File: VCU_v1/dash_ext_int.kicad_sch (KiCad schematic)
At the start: 33 parts, among them U15 SP8K80TB1, U16 SP8K80TB1

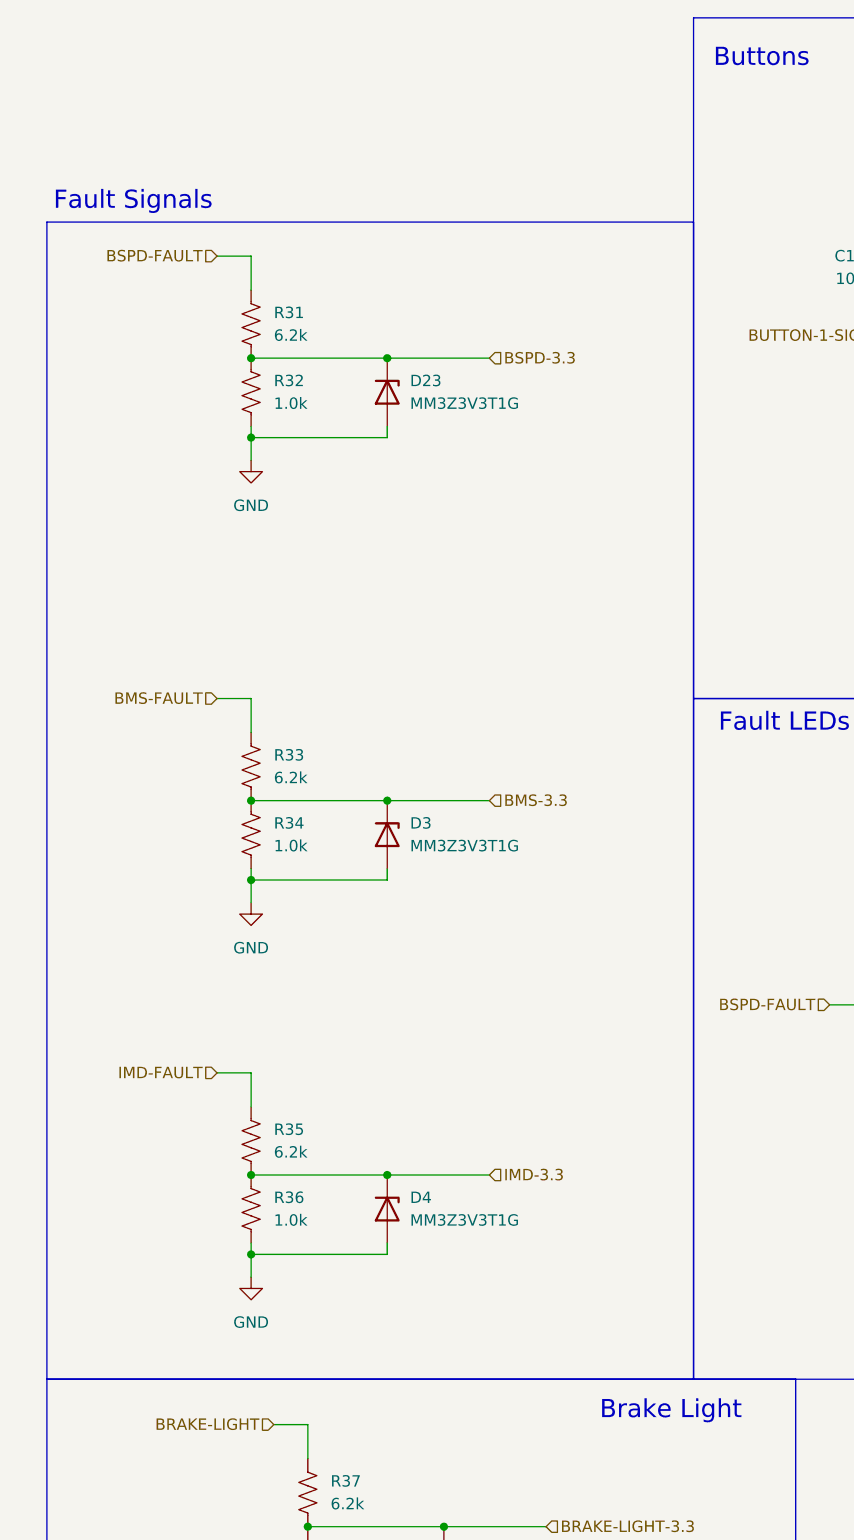
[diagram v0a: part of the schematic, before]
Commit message: left to do before layout: wire DRS/Debug LEDs to connector, add BRUHbus ports
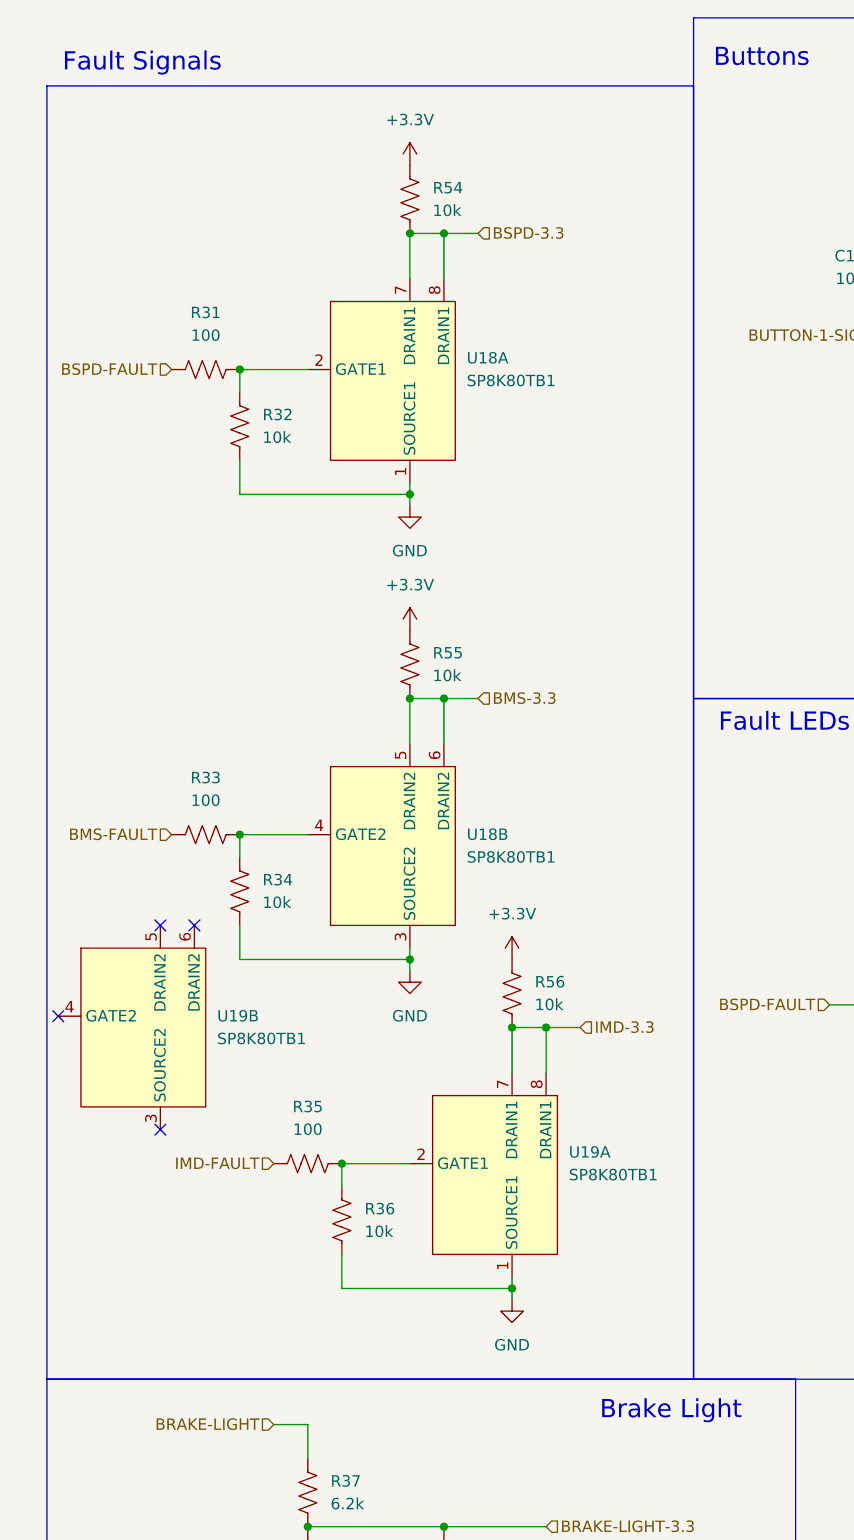
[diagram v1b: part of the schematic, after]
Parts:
- removed D23, D3, D4: MM3Z3V3T1G, Diode_SMD:D_SOD-323_HandSoldering, symbol .Diode-Zener:MM3Z3V3T1G
- removed R31, R33, R35: 6.2k, Resistor_SMD:R_0603_1608Metric_Pad0.98x0.95mm_HandSolder, symbol BFR Resistors:RMCF0603FT6K20
- removed R32, R34, R36: 1.0k, Resistor_SMD:R_0603_1608Metric_Pad0.98x0.95mm_HandSolder, symbol BFR Resistors:RMCF0603FT1K00
- added R31, R33, R35: 100, Resistor_SMD:R_0603_1608Metric_Pad0.98x0.95mm_HandSolder, symbol BFR Resistors:RMCF0603FT100R
- added R32, R34, R36, R54, R55, R56: 10k, Resistor_SMD:R_0603_1608Metric_Pad0.98x0.95mm_HandSolder, symbol BFR Resistors:RMCF0603FT10K0
- added U18, U19: SP8K80TB1, symbol SP8KK80TB1:SP8K80TB1
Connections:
- net BMS-3.3: now also R55.1, U18.5 (DRAIN2), U18.6 (DRAIN2)
- net BMS-FAULT: now also R33.1
- net BSPD-3.3: now also R54.1, U18.7 (DRAIN1), U18.8 (DRAIN1)
- net BSPD-FAULT: now also R31.1
- net GND: now also R32.1, R34.1, R36.1, U18.1 (SOURCE1), U18.3 (SOURCE2), U19.1 (SOURCE1)
- net IMD-3.3: now also R56.1, U19.7 (DRAIN1), U19.8 (DRAIN1)
- net IMD-FAULT: now also R35.1
- new net: R33.2, R34.2, U18.4 (GATE2)
- new net: R31.2, R32.2, U18.2 (GATE1)
- new net: R35.2, R36.2, U19.2 (GATE1)
- new net +3.3V: R54.2, R55.2, R56.2
- no-connect marks 4 -> 8
